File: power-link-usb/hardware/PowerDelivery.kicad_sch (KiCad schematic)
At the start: 22 parts, among them J201 DX07S016JA3, J202 KitProg3, Q201 BSC010N04LS, Q202 BSC010N04LS, U201 CYPM1311-48LDXI

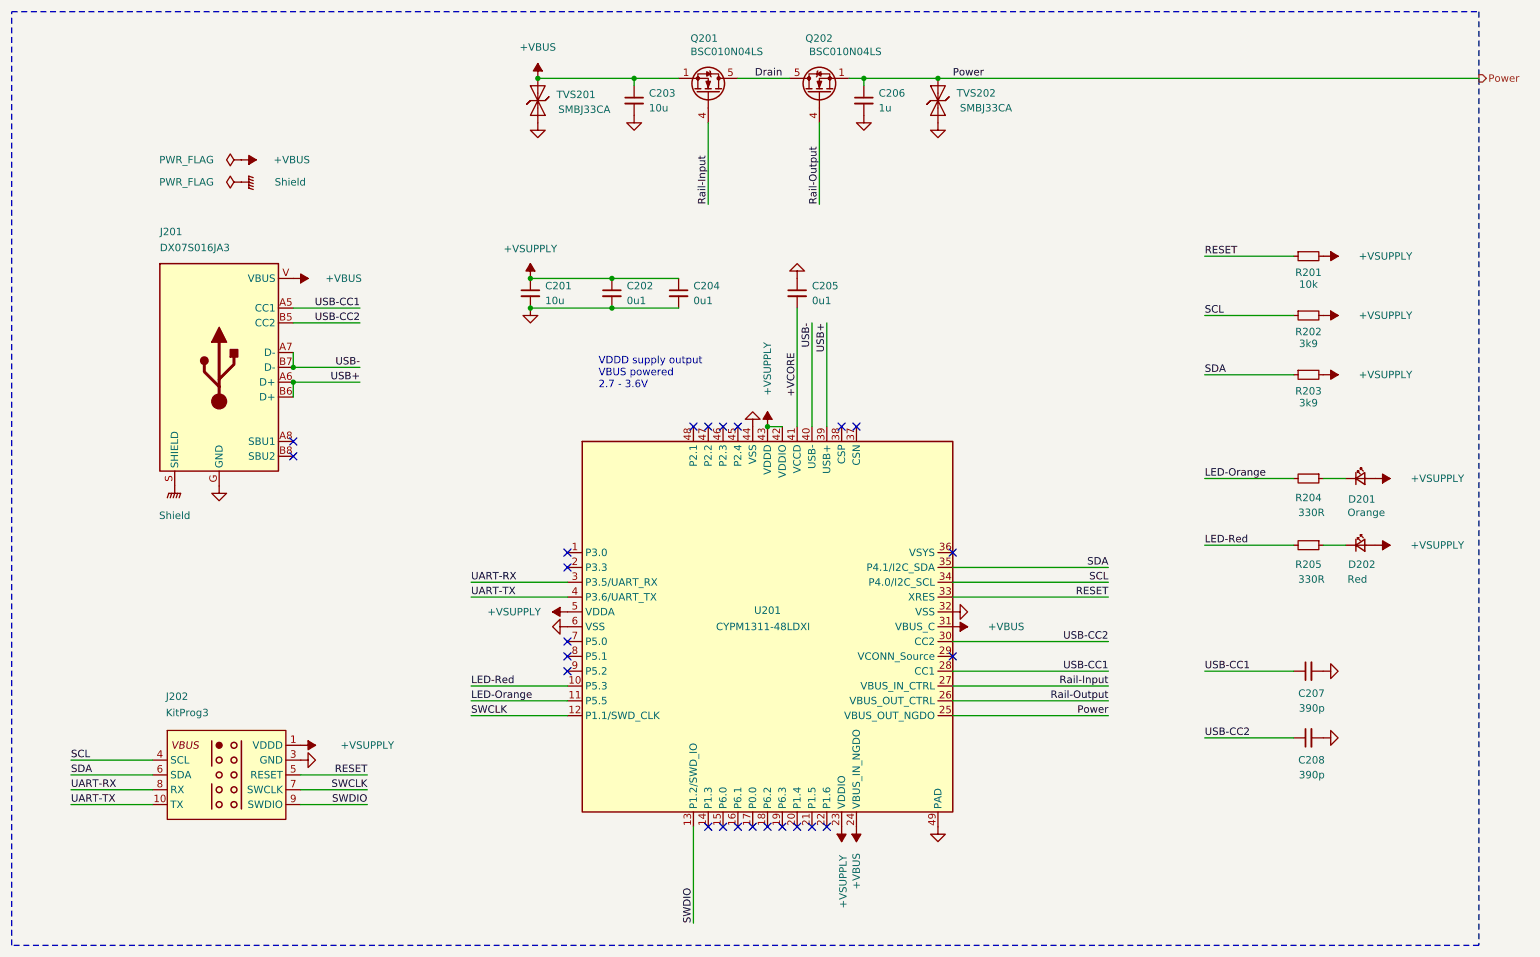
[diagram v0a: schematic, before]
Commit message: Update
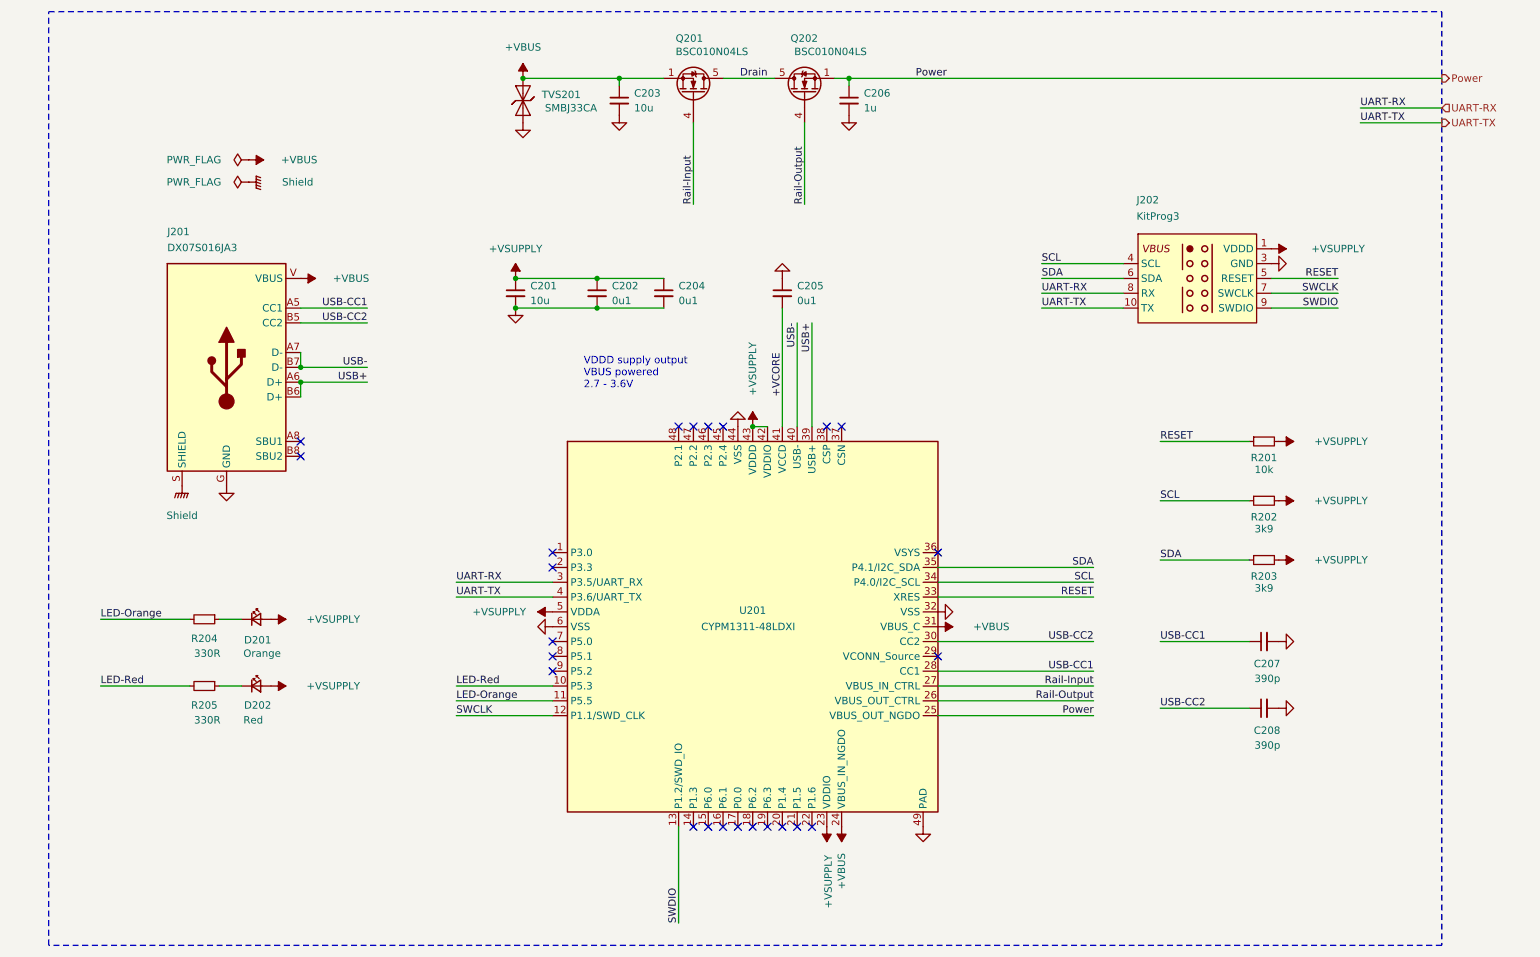
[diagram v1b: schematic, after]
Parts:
- removed TVS202: SMBJ33CA, V2_Diode_SMD:D_SMB, symbol V2_Diode:SMBJ33CA
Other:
- moved on the sheet: C201, C202, C203, C204, C205, C206, C207, C208, D201, D202, J201, J202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
